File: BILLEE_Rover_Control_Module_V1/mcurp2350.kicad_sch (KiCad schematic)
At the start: 53 parts, among them J1 2.54mm Header, SW2 KMR2, SW3 RESET SW, U15 W25Q128JVSIQTR, U16 SN74LVC244APWR, U17 ABM8-272-T3_C20625731, U18 RP2350A_C42411118, U19 SN74LVC244APWR, U21 TCA4307DGKR, U22 TCA4307DGKR

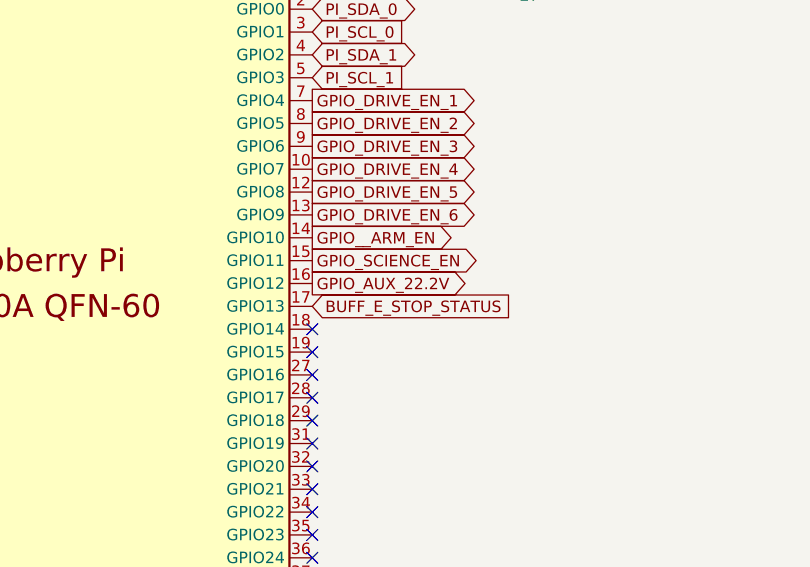
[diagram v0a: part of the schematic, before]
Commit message: WIP Checkpoint
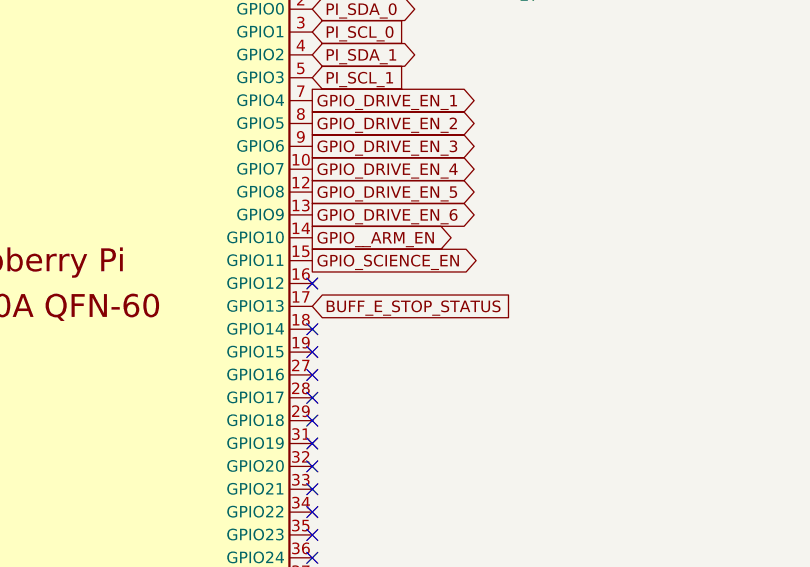
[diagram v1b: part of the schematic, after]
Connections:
- net GPIO_AUX_22.2V: no longer U18.16 (GPIO12)
- no-connect marks 33 -> 34
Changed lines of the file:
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@@
+	)
+	(no_connect
+		(at 151.13 114.3)
 	)
 	(no_connect
@@
 			)
 		)
-	)
-	(global_label "GPIO_AUX_22.2V"
-		(shape output)
-		(at 151.13 114.3 0)
-		(fields_autoplaced yes)
-		(effects
-			(font
-				(size 1.27 1.27)
-			)
-			(justify left)
-		)
-		(property "Intersheetrefs" "${INTERSHEET_REFS}"
-			(at 169.4762 114.3 0)
-			(hide yes)
-			(show_name no)
-			(do_not_autoplace no)
-			(effects
-				(font
-					(size 1.27 1.27)
-				)
-				(justify left)
-			)
-		)
